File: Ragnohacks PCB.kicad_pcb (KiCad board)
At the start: 2 copper layers, 85.6 x 54 mm, 35 parts, among them J1 Conn_01x02, J2 Conn_01x18, J3 Conn_01x18, J4 USB_A, SW1 SW_Push, U1 RP2040, U2 W25Q128JVS, U3 LD1117S33TR_SOT223, U4 USBLC6-2P6, Y1 12MHz

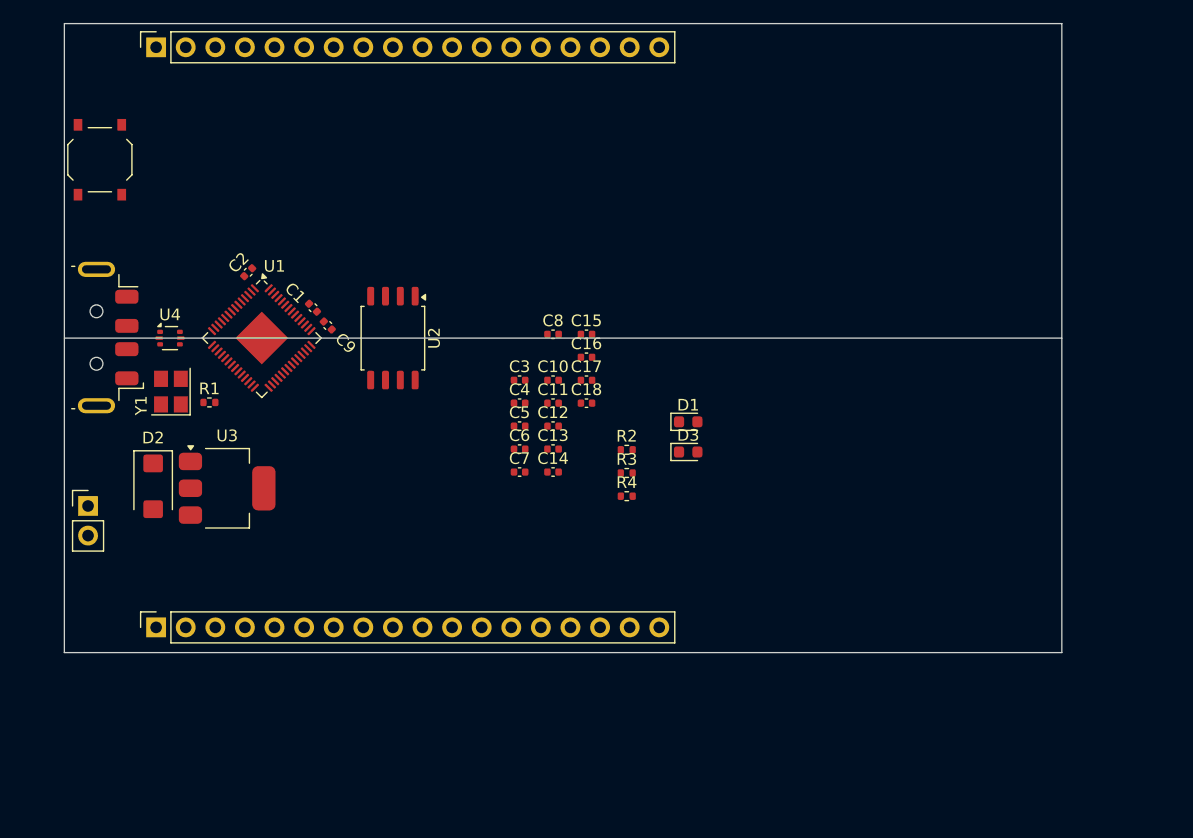
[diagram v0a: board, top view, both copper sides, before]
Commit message: Start tracing
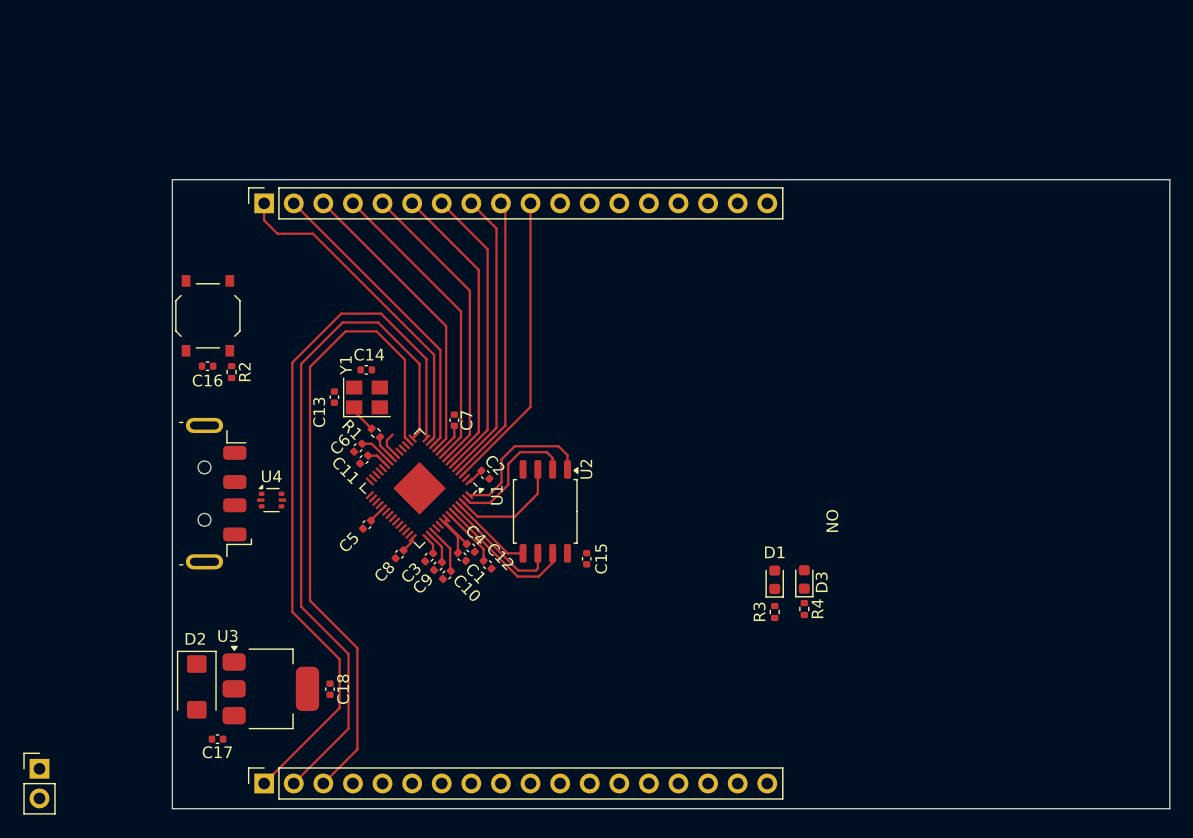
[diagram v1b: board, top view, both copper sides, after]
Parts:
- moved C17 44.2 mm to (107.4, 125.4), turned to 180 degrees
- moved R2 34.6 mm to (108.6, 93.9), turned to -90 degrees
- moved C18 33.0 mm to (117.0, 121.1), turned to -90 degrees
- moved C16 32.5 mm to (106.5, 93.4)
- moved C2 26.8 mm to (130.4, 102.7), turned to -45 degrees
- moved C1 24.9 mm to (128.3, 109.8)
- moved C8 23.0 mm to (123.0, 109.6), turned to -135 degrees
- moved J1 22.9 mm to (92.1, 128.0)
- moved C9 22.7 mm to (126.3, 110.6), turned to -135 degrees
- moved U2 19.8 mm to (135.5, 105.9)
- moved C13 19.3 mm to (117.4, 96.1), turned to -90 degrees
- moved C15 19.3 mm to (139.1, 109.9), turned to 90 degrees
- moved C10 19.0 mm to (127.1, 111.3), turned to -135 degrees
- moved U1 18.7 mm to (124.7, 103.9), turned to -135 degrees
- moved C14 18.3 mm to (120.1, 93.7)
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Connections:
- U1 pad 14: D14 -> D0
- U1 pad 15: D13 -> D1
- U1 pad 16: D12 -> D2
- U1 pad 17: D11 -> D3
- U1 pad 18: D10 -> D4
- U1 pad 27: D9 -> D5
- U1 pad 28: D8 -> D6
- U1 pad 30: D6 -> D8
- U1 pad 31: D5 -> D9
- U1 pad 32: D4 -> D10
- U1 pad 34: D3 -> D11
- U1 pad 35: D2 -> D12
- U1 pad 36: D1 -> D13
- U1 pad 37: D0 -> D14
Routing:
- net D0: track 0.00 -> 62.2 mm
- net D1: track 0.00 -> 59.4 mm
- net D2: track 0.00 -> 56.3 mm
- net D15: track 0.00 -> 28.4 mm
- net D16: track 0.00 -> 26.2 mm
- net D18: track 0.00 -> 26.1 mm
- net D19: track 0.00 -> 25.8 mm
- net D17: track 0.00 -> 25.7 mm
- net D24: track 0.00 -> 25.7 mm
- net D20: track 0.00 -> 25.6 mm
- net D21: track 0.00 -> 25.3 mm
- net D22: track 0.00 -> 25.1 mm
- net D23: track 0.00 -> 24.8 mm
- net +3V3: track 0.00 -> 20.5 mm
- net FLASH_CS: track 0.00 -> 12.9 mm
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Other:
- outline, holes or cut-outs redrawn
- board text added: "ON"
